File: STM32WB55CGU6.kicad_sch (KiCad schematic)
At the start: 25 parts, among them IC2 STM32WB55CGU6, J11 BOOT0_Jumper, J9 Coin Battery Jumper, Y1 ABM3B-32.000MHZ-8-R30-B1U-T

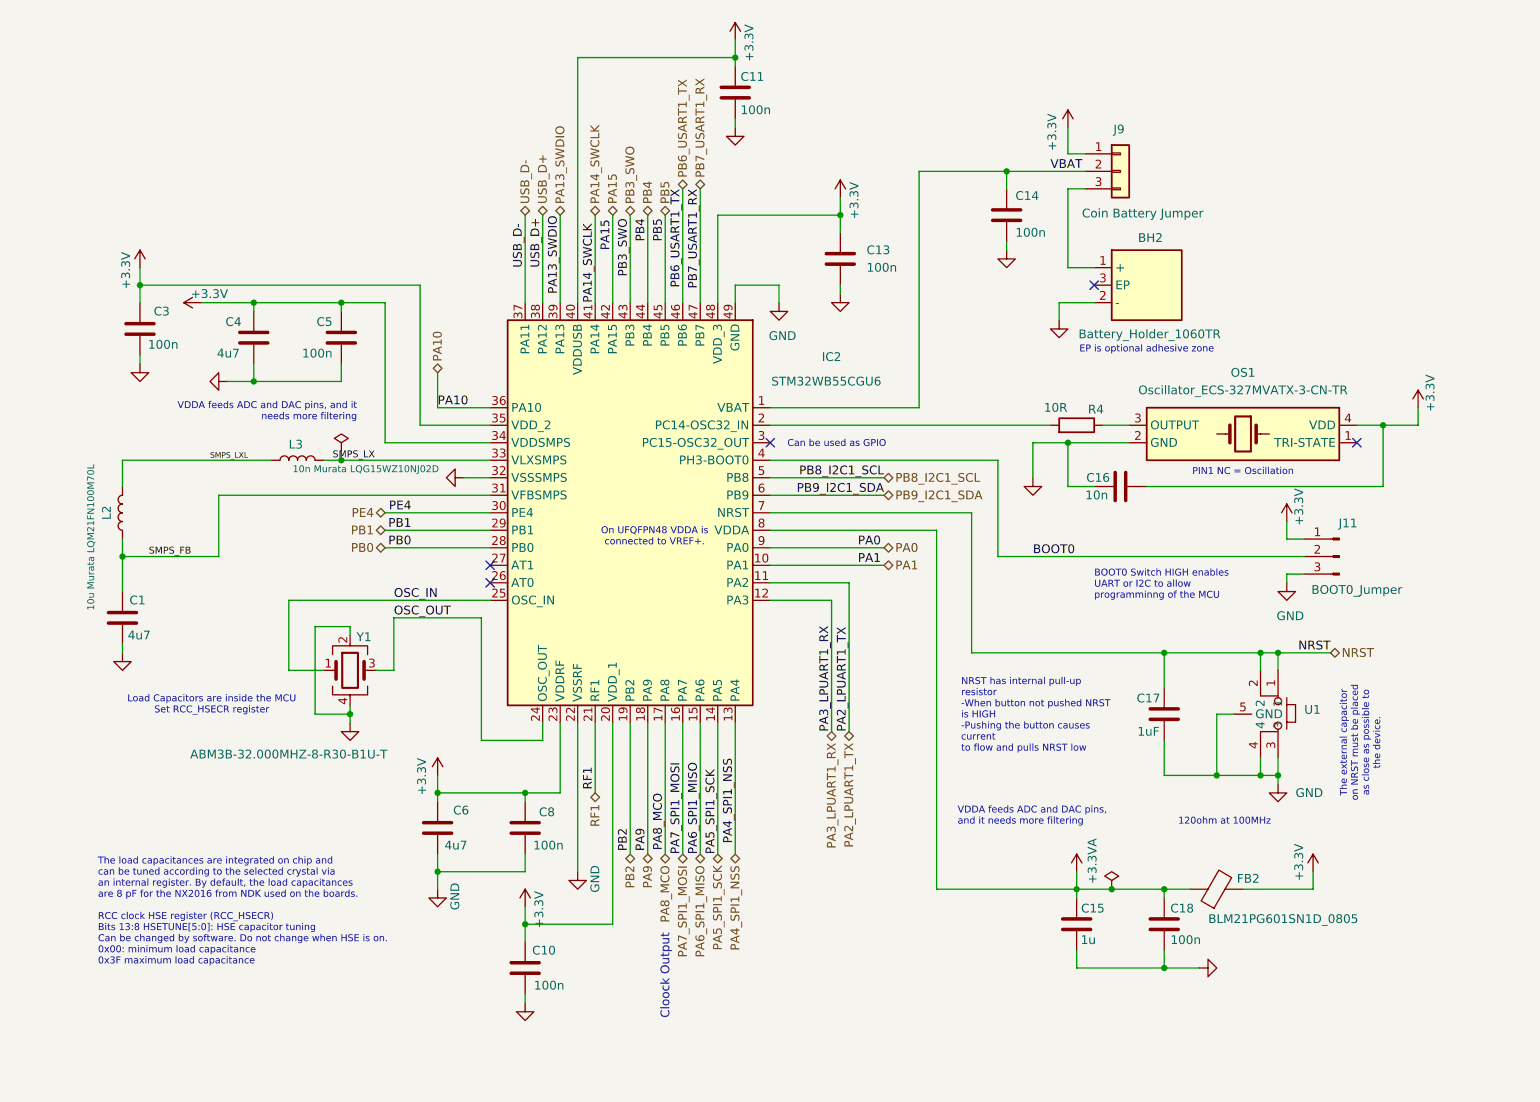
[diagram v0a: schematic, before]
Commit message: Update
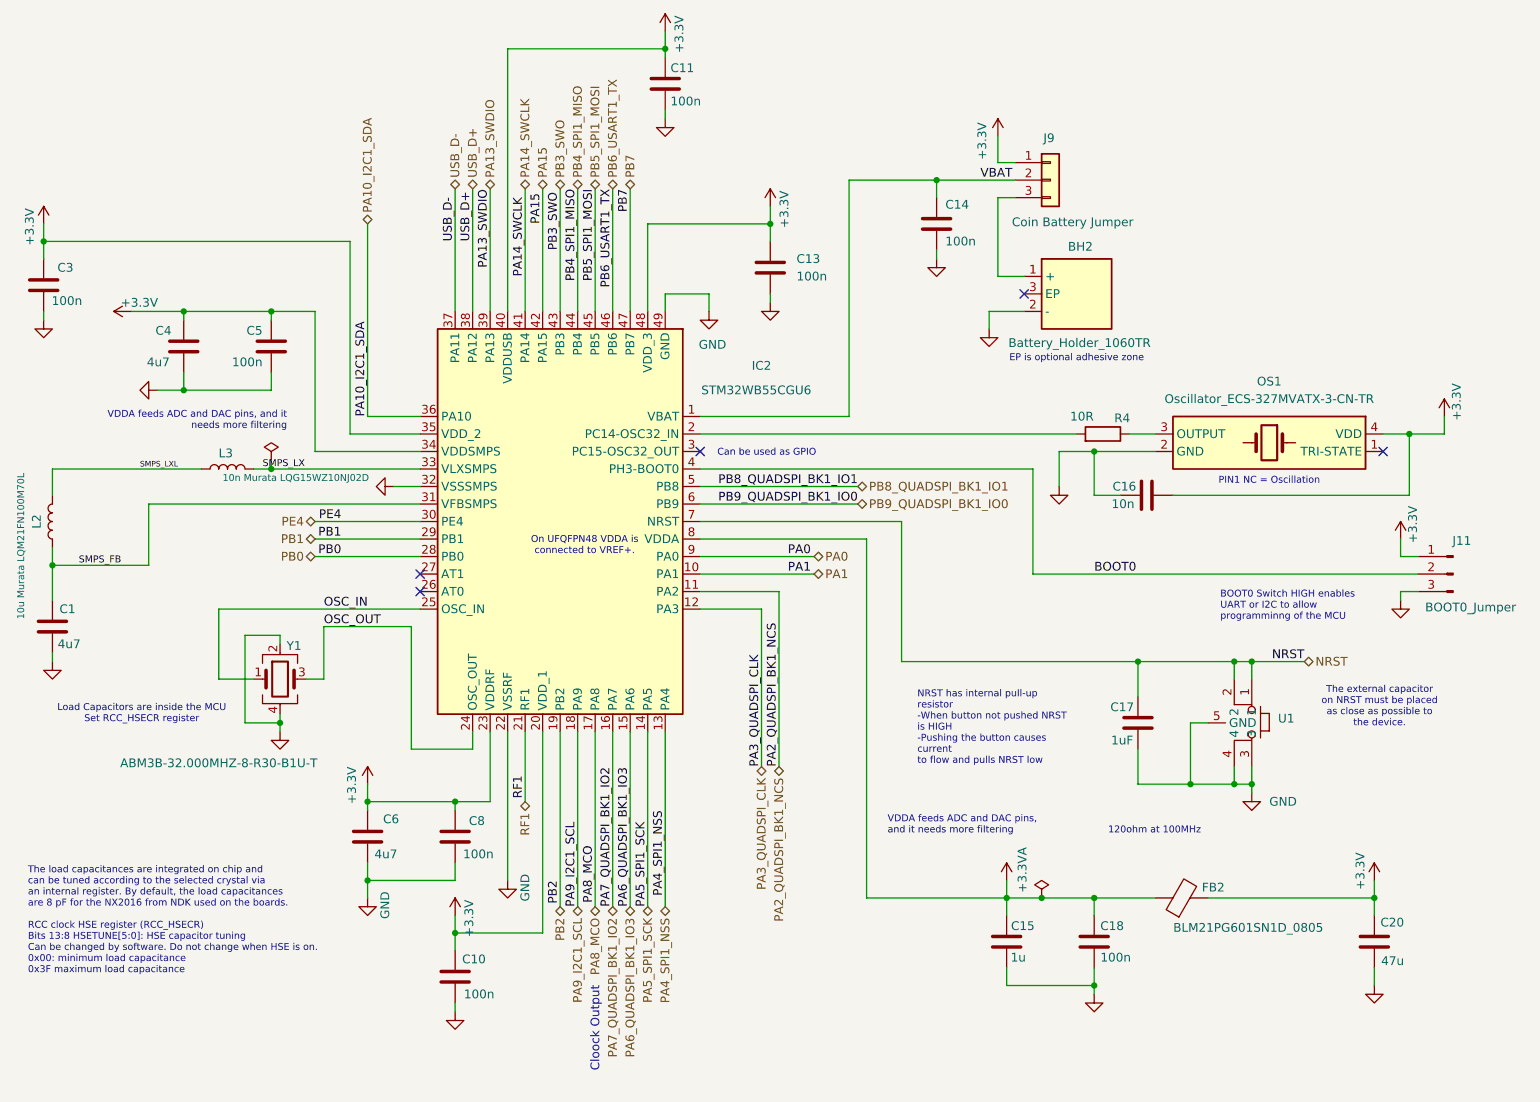
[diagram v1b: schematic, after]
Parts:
- added C20: 47u, Capacitor_SMD:C_0805_2012Metric, symbol Device:C
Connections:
- net +3.3V: now also C20.1
- net GND: now also C20.2
- net PA10 renamed PA10_I2C1_SDA
- net PA2_LPUART1_TX renamed PA2_QUADSPI_BK1_NCS
- net PA3_LPUART1_RX renamed PA3_QUADSPI_CLK
- net PA6_SPI1_MISO renamed PA6_QUADSPI_BK1_IO3
- net PA7_SPI1_MOSI renamed PA7_QUADSPI_BK1_IO2
- net PA9 renamed PA9_I2C1_SCL
- net PB4 renamed PB4_SPI1_MISO
- net PB5 renamed PB5_SPI1_MOSI
- net PB7_USART1_RX renamed PB7
- net PB8_I2C1_SCL renamed PB8_QUADSPI_BK1_IO1
- net PB9_I2C1_SDA renamed PB9_QUADSPI_BK1_IO0
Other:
- company: (none) -> Peter Hancak
- title: (none) -> Bluetooth_STM32WB55_Board
- moved on the sheet: BH2, C1, C10, C11, C13, C14, C15, C16, C17, C18, C3, C4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

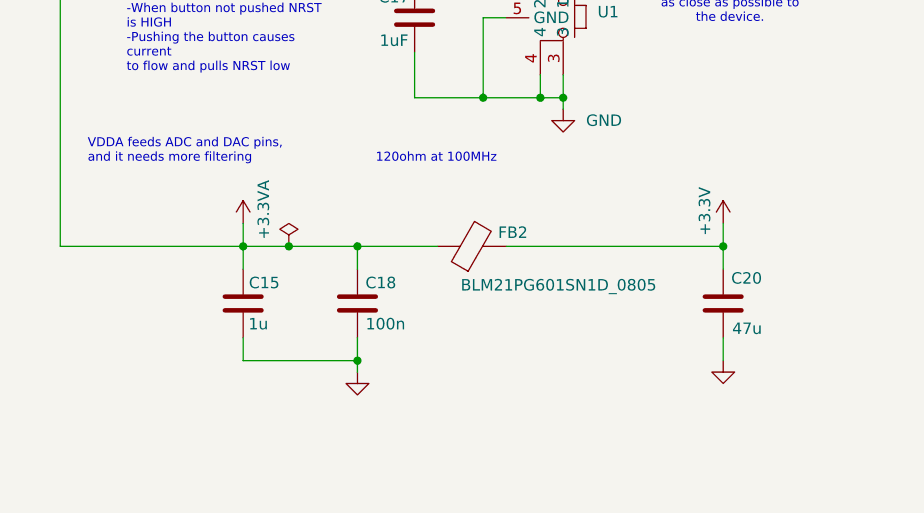
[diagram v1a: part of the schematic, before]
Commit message: Update
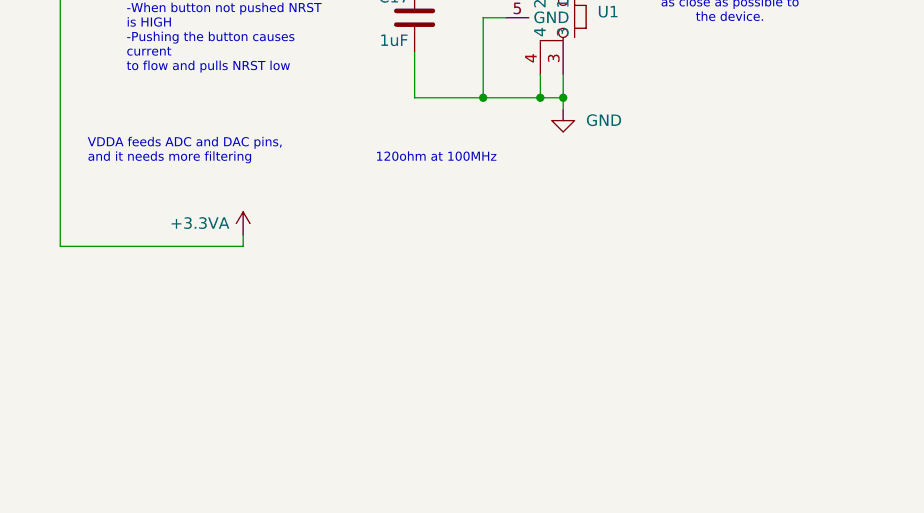
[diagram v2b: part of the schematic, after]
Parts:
- removed C15: 1u, Capacitor_SMD:C_0805_2012Metric, symbol Device:C
- removed C18: 100n, Capacitor_SMD:C_0805_2012Metric, symbol Device:C
- removed C20: 47u, Capacitor_SMD:C_0805_2012Metric, symbol Device:C
- removed FB2: BLM21PG601SN1D_0805, Capacitor_SMD:C_0805_2012Metric, symbol Device:FerriteBead
